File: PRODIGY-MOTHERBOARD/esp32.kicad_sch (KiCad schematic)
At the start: 13 parts, among them J24 Bus_M.2_Socket_B, J25 USB_C_Receptacle, SW2 SW_Push

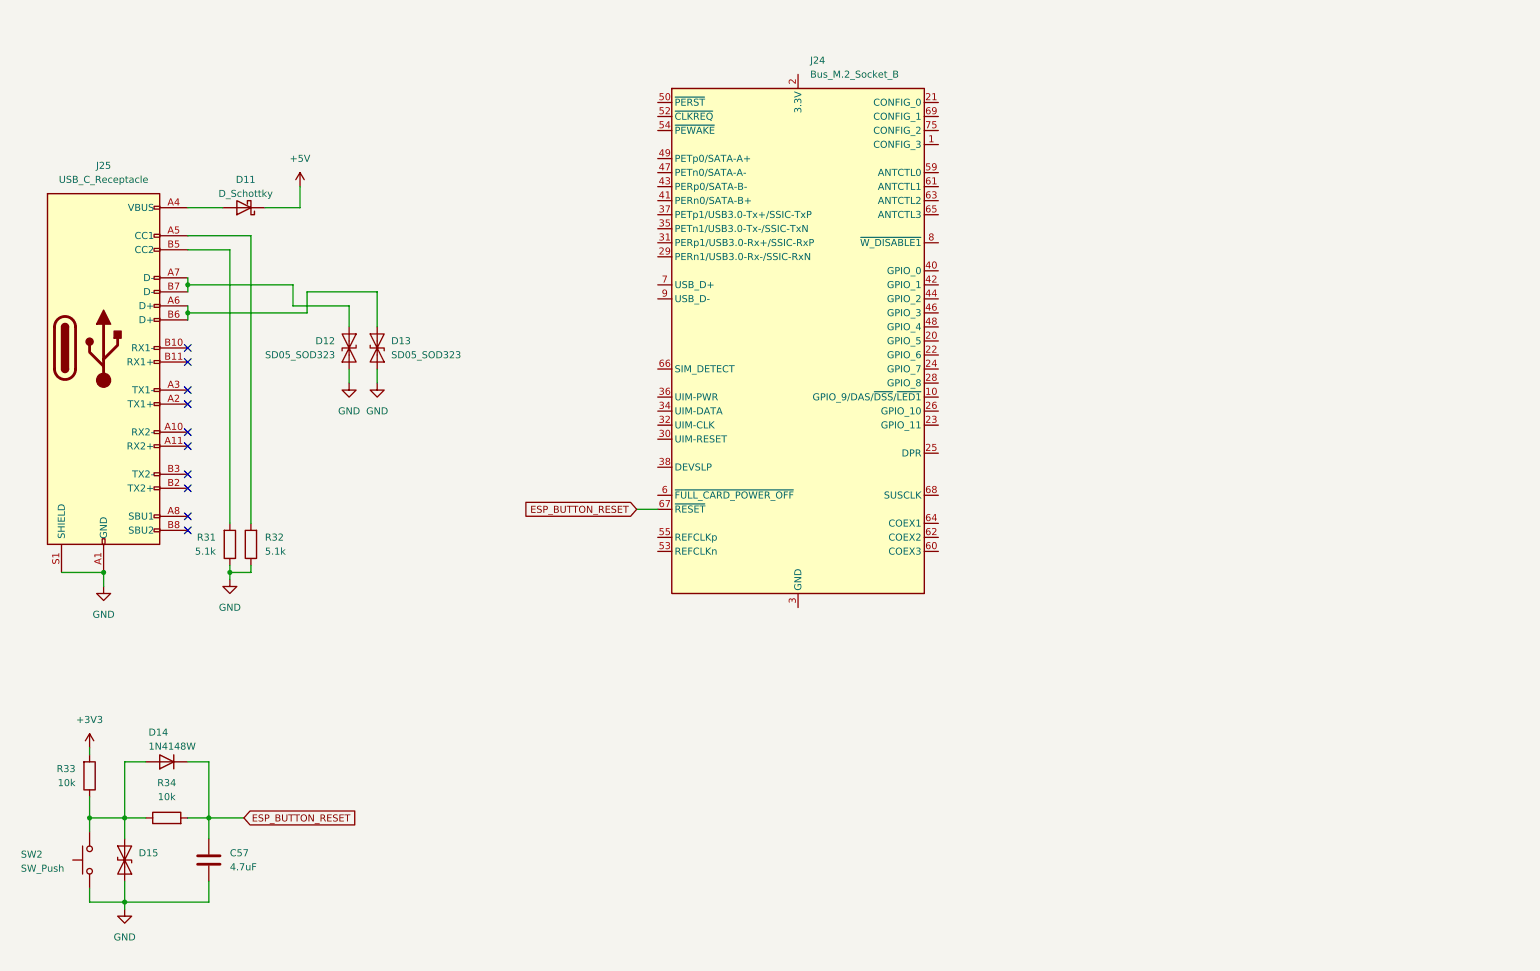
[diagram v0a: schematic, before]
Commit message: Esp32 motherboard schematic done.
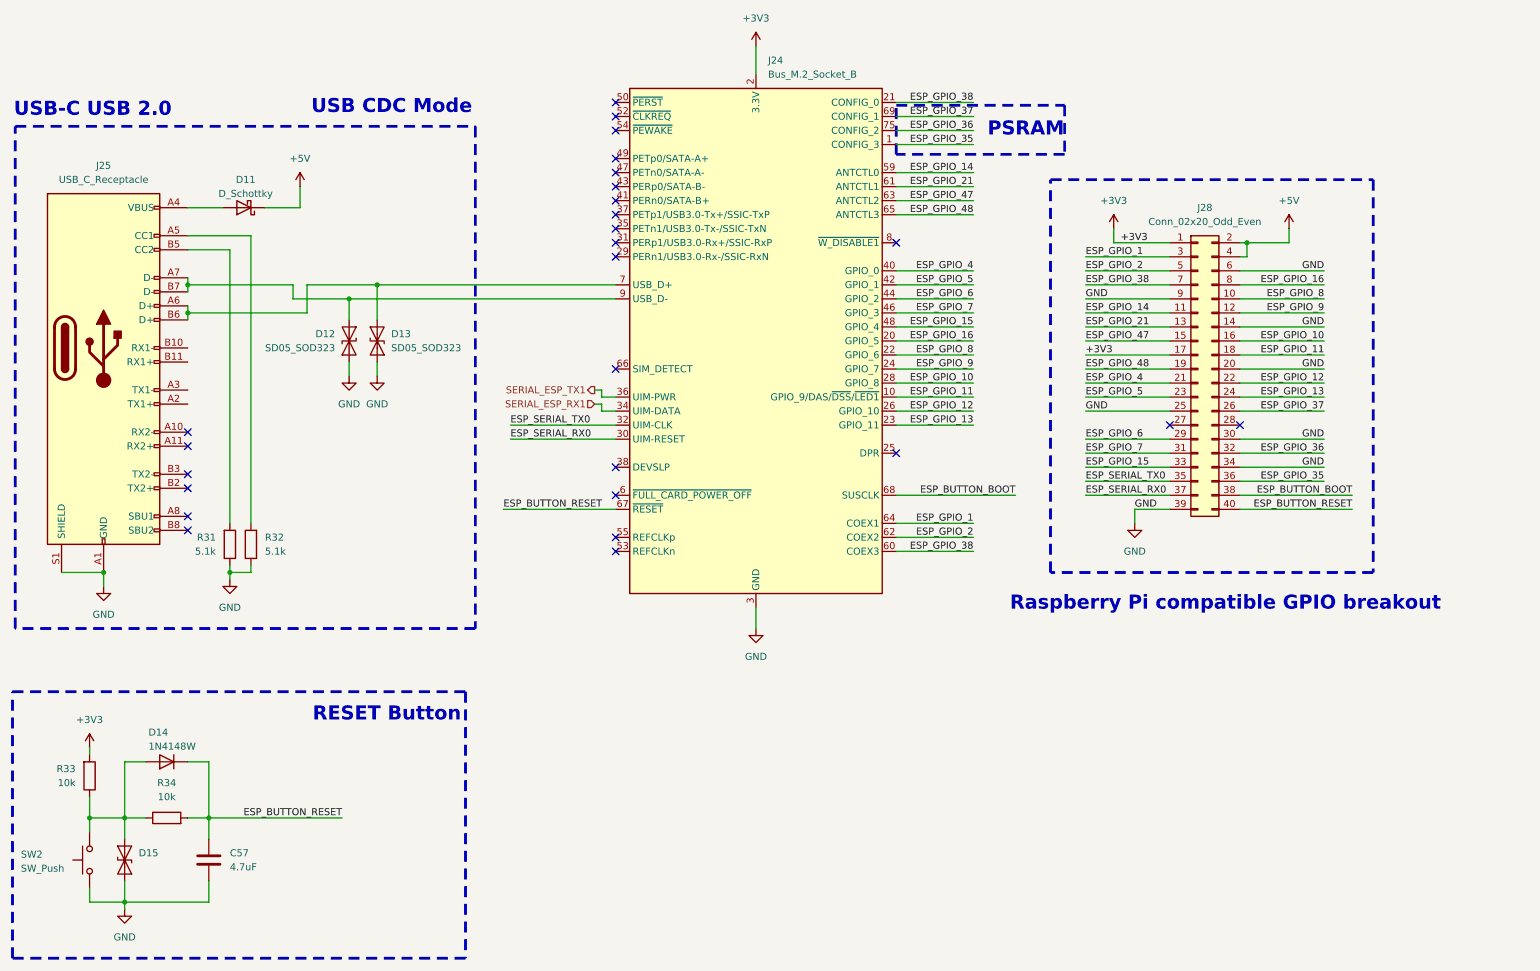
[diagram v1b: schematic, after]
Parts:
- added J28: Conn_02x20_Odd_Even, Connector_PinHeader_2.54mm:PinHeader_2x20_P2.54mm_Horizontal, symbol Connector_Generic:Conn_02x20_Odd_Even
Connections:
- net +3V3: now also J24.2 (3.3V), J24.4 (3.3V), J24.70 (3.3V), J24.72 (3.3V), J24.74 (3.3V), J28.1 (Pin_1), J28.17 (Pin_17)
- net +5V: now also J28.2 (Pin_2), J28.4 (Pin_4)
- net ESP_BUTTON_RESET: now also J28.40 (Pin_40)
- net GND: now also J24.11 (GND), J24.27 (GND), J24.3 (GND), J24.33 (GND), J24.39 (GND), J24.45 (GND), J24.5 (GND), J24.51 (GND), J24.57 (GND), J24.71 (GND), J24.73 (GND), J28.14 (Pin_14), J28.20 (Pin_20), J28.25 (Pin_25), J28.30 (Pin_30), J28.34 (Pin_34), J28.39 (Pin_39), J28.6 (Pin_6), J28.9 (Pin_9)
- net at D13.2 (A2), J25.A6 (D+), J25.B6 (D+): now also J24.7 (USB_D+)
- net at D12.2 (A2), J25.A7 (D-), J25.B7 (D-): now also J24.9 (USB_D-)
- net ESP_GPIO_35: now reaches J24.1 (CONFIG_3)
- net ESP_GPIO_35: now also J28.36 (Pin_36)
- net ESP_GPIO_11: now reaches J24.10 (GPIO_9/DAS/~{DSS}/~{LED1})
- net ESP_GPIO_11: now also J28.18 (Pin_18)
- net ESP_GPIO_16: now reaches J24.20 (GPIO_5)
- net ESP_GPIO_16: now also J28.8 (Pin_8)
- net ESP_GPIO_38: now reaches J24.21 (CONFIG_0)
- net ESP_GPIO_38: now also J24.60 (COEX3), J28.7 (Pin_7)
- net ESP_GPIO_8: now reaches J24.22 (GPIO_6)
- net ESP_GPIO_8: now also J28.10 (Pin_10)
- net ESP_GPIO_13: now reaches J24.23 (GPIO_11)
- net ESP_GPIO_13: now also J28.24 (Pin_24)
- net ESP_GPIO_9: now reaches J24.24 (GPIO_7)
- net ESP_GPIO_9: now also J28.12 (Pin_12)
- net ESP_GPIO_12: now reaches J24.26 (GPIO_10)
- net ESP_GPIO_12: now also J28.22 (Pin_22)
- net ESP_GPIO_10: now reaches J24.28 (GPIO_8)
- net ESP_GPIO_10: now also J28.16 (Pin_16)
- net ESP_SERIAL_RX0: now reaches J24.30 (UIM-RESET)
- net ESP_SERIAL_RX0: now also J28.37 (Pin_37)
- net ESP_SERIAL_TX0: now reaches J24.32 (UIM-CLK)
- net ESP_SERIAL_TX0: now also J28.35 (Pin_35)
- net SERIAL_ESP_RX1: now reaches J24.34 (UIM-DATA)
- net SERIAL_ESP_TX1: now reaches J24.36 (UIM-PWR)
- net ESP_GPIO_4: now reaches J24.40 (GPIO_0)
- net ESP_GPIO_4: now also J28.21 (Pin_21)
- net ESP_GPIO_5: now reaches J24.42 (GPIO_1)
- net ESP_GPIO_5: now also J28.23 (Pin_23)
- net ESP_GPIO_6: now reaches J24.44 (GPIO_2)
- net ESP_GPIO_6: now also J28.29 (Pin_29)
- net ESP_GPIO_7: now reaches J24.46 (GPIO_3)
- net ESP_GPIO_7: now also J28.31 (Pin_31)
- net ESP_GPIO_15: now reaches J24.48 (GPIO_4)
- net ESP_GPIO_15: now also J28.33 (Pin_33)
- net ESP_GPIO_14: now reaches J24.59 (ANTCTL0)
- net ESP_GPIO_14: now also J28.11 (Pin_11)
- net ESP_GPIO_21: now reaches J24.61 (ANTCTL1)
- net ESP_GPIO_21: now also J28.13 (Pin_13)
- net ESP_GPIO_2: now reaches J24.62 (COEX2)
- net ESP_GPIO_2: now also J28.5 (Pin_5)
- net ESP_GPIO_47: now reaches J24.63 (ANTCTL2)
- net ESP_GPIO_47: now also J28.15 (Pin_15)
- net ESP_GPIO_1: now reaches J24.64 (COEX1)
- net ESP_GPIO_1: now also J28.3 (Pin_3)
- net ESP_GPIO_48: now reaches J24.65 (ANTCTL3)
- net ESP_GPIO_48: now also J28.19 (Pin_19)
- net ESP_BUTTON_BOOT: now reaches J24.68 (SUSCLK)
- net ESP_BUTTON_BOOT: now also J28.38 (Pin_38)
- net ESP_GPIO_37: now reaches J24.69 (CONFIG_1)
- net ESP_GPIO_37: now also J28.26 (Pin_26)
- net ESP_GPIO_36: now reaches J24.75 (CONFIG_2)
- net ESP_GPIO_36: now also J28.32 (Pin_32)
- no-connect marks 10 -> 26
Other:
- note added: "PSRAM"
- note added: "RESET Button"
- note added: "Raspberry Pi compatible GPIO breakout"
- note added: "USB CDC Mode"
- note added: "USB-C USB 2.0"
- moved on the sheet: J24
